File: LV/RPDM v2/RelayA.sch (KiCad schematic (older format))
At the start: 6 parts, among them K2 G8NW, Q3 Q_Dual_NMOS

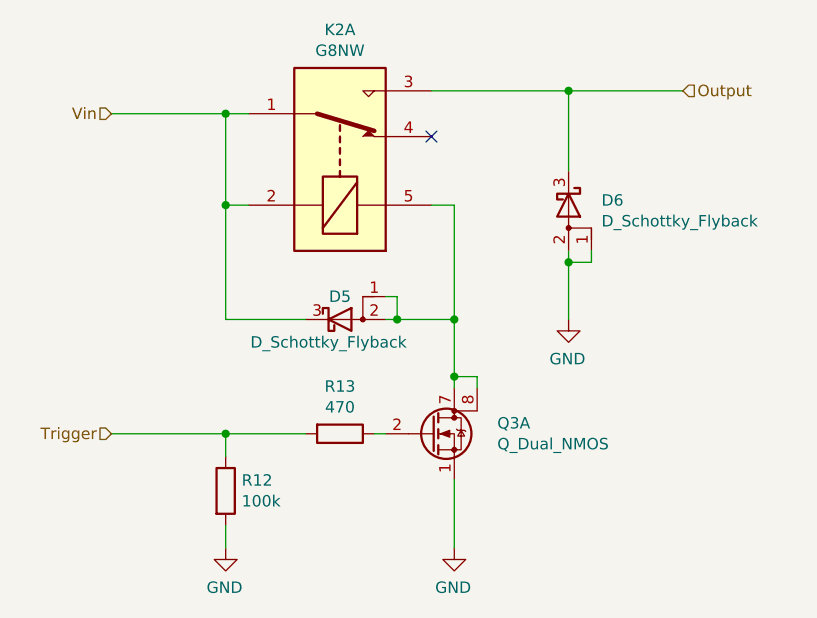
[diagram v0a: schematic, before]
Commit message: RPDM nearly finished
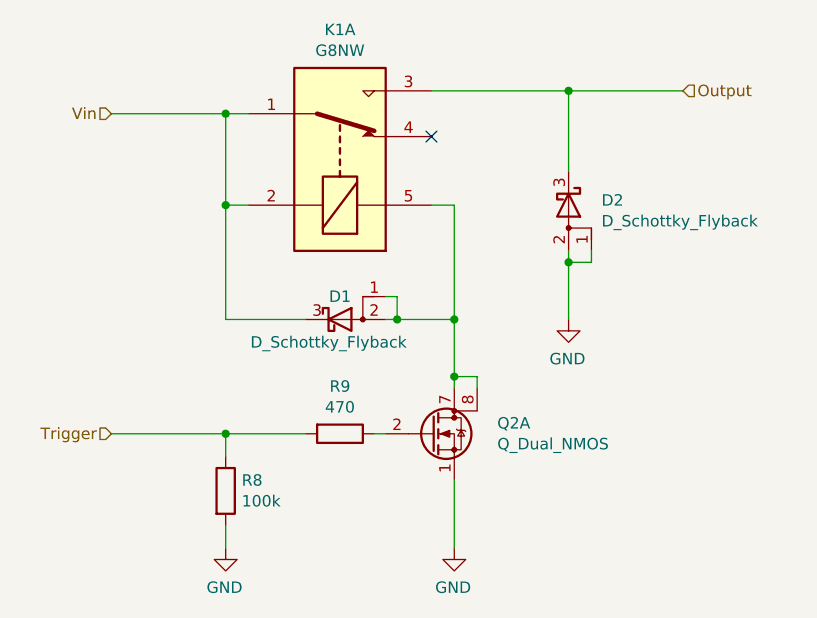
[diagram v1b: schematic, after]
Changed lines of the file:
@@
 $Descr A4 11693 8268
 encoding utf-8
-Sheet 29 30
+Sheet 27 30
 Title "Relay Circuit"
 Date "2021-06-28"
@@
 AR Path="/5E554D5D/60DE88EB/6183CC28" Ref="R?"  Part="1"
 AR Path="/5E554D5D/60DEDCB5/6183CC28" Ref="R?"  Part="1"
-F 0 "R12" H 5070 4796 50  0000 L CNN
+F 0 "R8" H 5070 4796 50  0000 L CNN
 F 1 "100k" H 5070 4705 50  0000 L CNN
 F 2 "Resistor_SMD:R_0805_2012Metric_Pad1.15x1.40mm_HandSolder" V 4930 4750 50  0001 C CNN
@@
 AR Path="/5E554D5D/60DE88EB/6114E9D1" Ref="Q?"  Part="1"
 AR Path="/5E554D5D/60DED789/6114E9D1" Ref="Q2"  Part="1"
-F 0 "Q3" H 6188 4546 50  0000 L CNN
+F 0 "Q2" H 6188 4546 50  0000 L CNN
 F 1 "Q_Dual_NMOS" H 6188 4455 50  0000 L CNN
 F 2 "UOWM_Package_SO:Diodes_SO-8_5.3x6.2mm_P1.27mm" H 6100 4500 50  0001 C CNN
@@
 AR Path="/5E554D5D/5E5E9CA9/61724099" Ref="K2"  Part="1"
 AR Path="/5E554D5D/60DED789/61724099" Ref="K1"  Part="1"
-F 0 "K2" V 6067 3300 50  0000 C CNN
+F 0 "K1" V 6067 3300 50  0000 C CNN
 F 1 "G8NW" V 5976 3300 50  0000 C CNN
 F 2 "UOWM_Relays:Omron-G8NW-2L-AS_SK-MFG" H 5900 3200 50  0001 L CNN
@@
 AR Path="/5E554D5D/5E5E9CA9/6174AD0B" Ref="R13"  Part="1"
 AR Path="/5E554D5D/60DED789/6174AD0B" Ref="R9"  Part="1"
-F 0 "R13" V 5293 4500 50  0000 C CNN
+F 0 "R9" V 5293 4500 50  0000 C CNN
 F 1 "470" V 5384 4500 50  0000 C CNN
 F 2 "Resistor_SMD:R_0805_2012Metric_Pad1.15x1.40mm_HandSolder" V 5430 4500 50  0001 C CNN
@@
 AR Path="/5E554D5D/60DED789/617CF33C" Ref="D1"  Part="1"
 AR Path="/5E554D5D/5E5E9CA9/617CF33C" Ref="D5"  Part="1"
-F 0 "D5" H 5500 4100 50  0000 C CNN
+F 0 "D1" H 5500 4100 50  0000 C CNN
 F 1 "D_Schottky_Flyback" H 5450 3900 50  0000 C CNN
 F 2 "UOWM_Diodes:TO-277_FSV10150V" H 5500 4000 50  0001 C CNN
@@
 AR Path="/5E554D5D/60DED789/617CFABC" Ref="D2"  Part="1"
 AR Path="/5E554D5D/5E5E9CA9/617CFABC" Ref="D6"  Part="1"
-F 0 "D6" V 6479 3644 50  0000 L CNN
+F 0 "D2" V 6479 3644 50  0000 L CNN
 F 1 "D_Schottky_Flyback" V 6570 3644 50  0000 L CNN
 F 2 "UOWM_Diodes:TO-277_FSV10150V" H 6500 3500 50  0001 C CNN

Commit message: RPDM
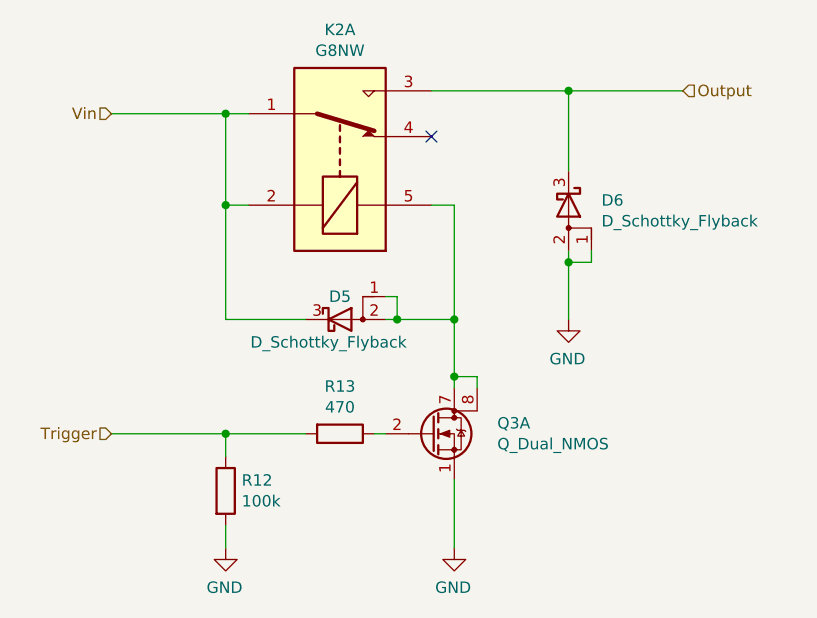
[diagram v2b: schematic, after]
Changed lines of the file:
@@
 $Descr A4 11693 8268
 encoding utf-8
-Sheet 27 30
+Sheet 29 30
 Title "Relay Circuit"
 Date "2021-06-28"
@@
 AR Path="/5E554D5D/60DE88EB/6183CC28" Ref="R?"  Part="1"
 AR Path="/5E554D5D/60DEDCB5/6183CC28" Ref="R?"  Part="1"
-F 0 "R8" H 5070 4796 50  0000 L CNN
+F 0 "R12" H 5070 4796 50  0000 L CNN
 F 1 "100k" H 5070 4705 50  0000 L CNN
 F 2 "Resistor_SMD:R_0805_2012Metric_Pad1.15x1.40mm_HandSolder" V 4930 4750 50  0001 C CNN
@@
 AR Path="/5E554D5D/60DE88EB/6114E9D1" Ref="Q?"  Part="1"
 AR Path="/5E554D5D/60DED789/6114E9D1" Ref="Q2"  Part="1"
-F 0 "Q2" H 6188 4546 50  0000 L CNN
+F 0 "Q3" H 6188 4546 50  0000 L CNN
 F 1 "Q_Dual_NMOS" H 6188 4455 50  0000 L CNN
 F 2 "UOWM_Package_SO:Diodes_SO-8_5.3x6.2mm_P1.27mm" H 6100 4500 50  0001 C CNN
@@
 AR Path="/5E554D5D/5E5E9CA9/61724099" Ref="K2"  Part="1"
 AR Path="/5E554D5D/60DED789/61724099" Ref="K1"  Part="1"
-F 0 "K1" V 6067 3300 50  0000 C CNN
+F 0 "K2" V 6067 3300 50  0000 C CNN
 F 1 "G8NW" V 5976 3300 50  0000 C CNN
 F 2 "UOWM_Relays:Omron-G8NW-2L-AS_SK-MFG" H 5900 3200 50  0001 L CNN
@@
 AR Path="/5E554D5D/5E5E9CA9/6174AD0B" Ref="R13"  Part="1"
 AR Path="/5E554D5D/60DED789/6174AD0B" Ref="R9"  Part="1"
-F 0 "R9" V 5293 4500 50  0000 C CNN
+F 0 "R13" V 5293 4500 50  0000 C CNN
 F 1 "470" V 5384 4500 50  0000 C CNN
 F 2 "Resistor_SMD:R_0805_2012Metric_Pad1.15x1.40mm_HandSolder" V 5430 4500 50  0001 C CNN
@@
 AR Path="/5E554D5D/60DED789/617CF33C" Ref="D1"  Part="1"
 AR Path="/5E554D5D/5E5E9CA9/617CF33C" Ref="D5"  Part="1"
-F 0 "D1" H 5500 4100 50  0000 C CNN
+F 0 "D5" H 5500 4100 50  0000 C CNN
 F 1 "D_Schottky_Flyback" H 5450 3900 50  0000 C CNN
 F 2 "UOWM_Diodes:TO-277_FSV10150V" H 5500 4000 50  0001 C CNN
@@
 AR Path="/5E554D5D/60DED789/617CFABC" Ref="D2"  Part="1"
 AR Path="/5E554D5D/5E5E9CA9/617CFABC" Ref="D6"  Part="1"
-F 0 "D2" V 6479 3644 50  0000 L CNN
+F 0 "D6" V 6479 3644 50  0000 L CNN
 F 1 "D_Schottky_Flyback" V 6570 3644 50  0000 L CNN
 F 2 "UOWM_Diodes:TO-277_FSV10150V" H 6500 3500 50  0001 C CNN
